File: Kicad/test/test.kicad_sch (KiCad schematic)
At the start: 74 parts, among them J1 SPKOUT, J2 Tag Con, P1 USB_C_Plug_USB2.0, SW1 SW_Push, SW2 SW_Push, SW4 SW_Push, SW5 SW_Push, U1 MAX98357A, U2 ESP32-S3-WROOM-1, U3 OV5640, U4 24Mhz, U5 AXP2101

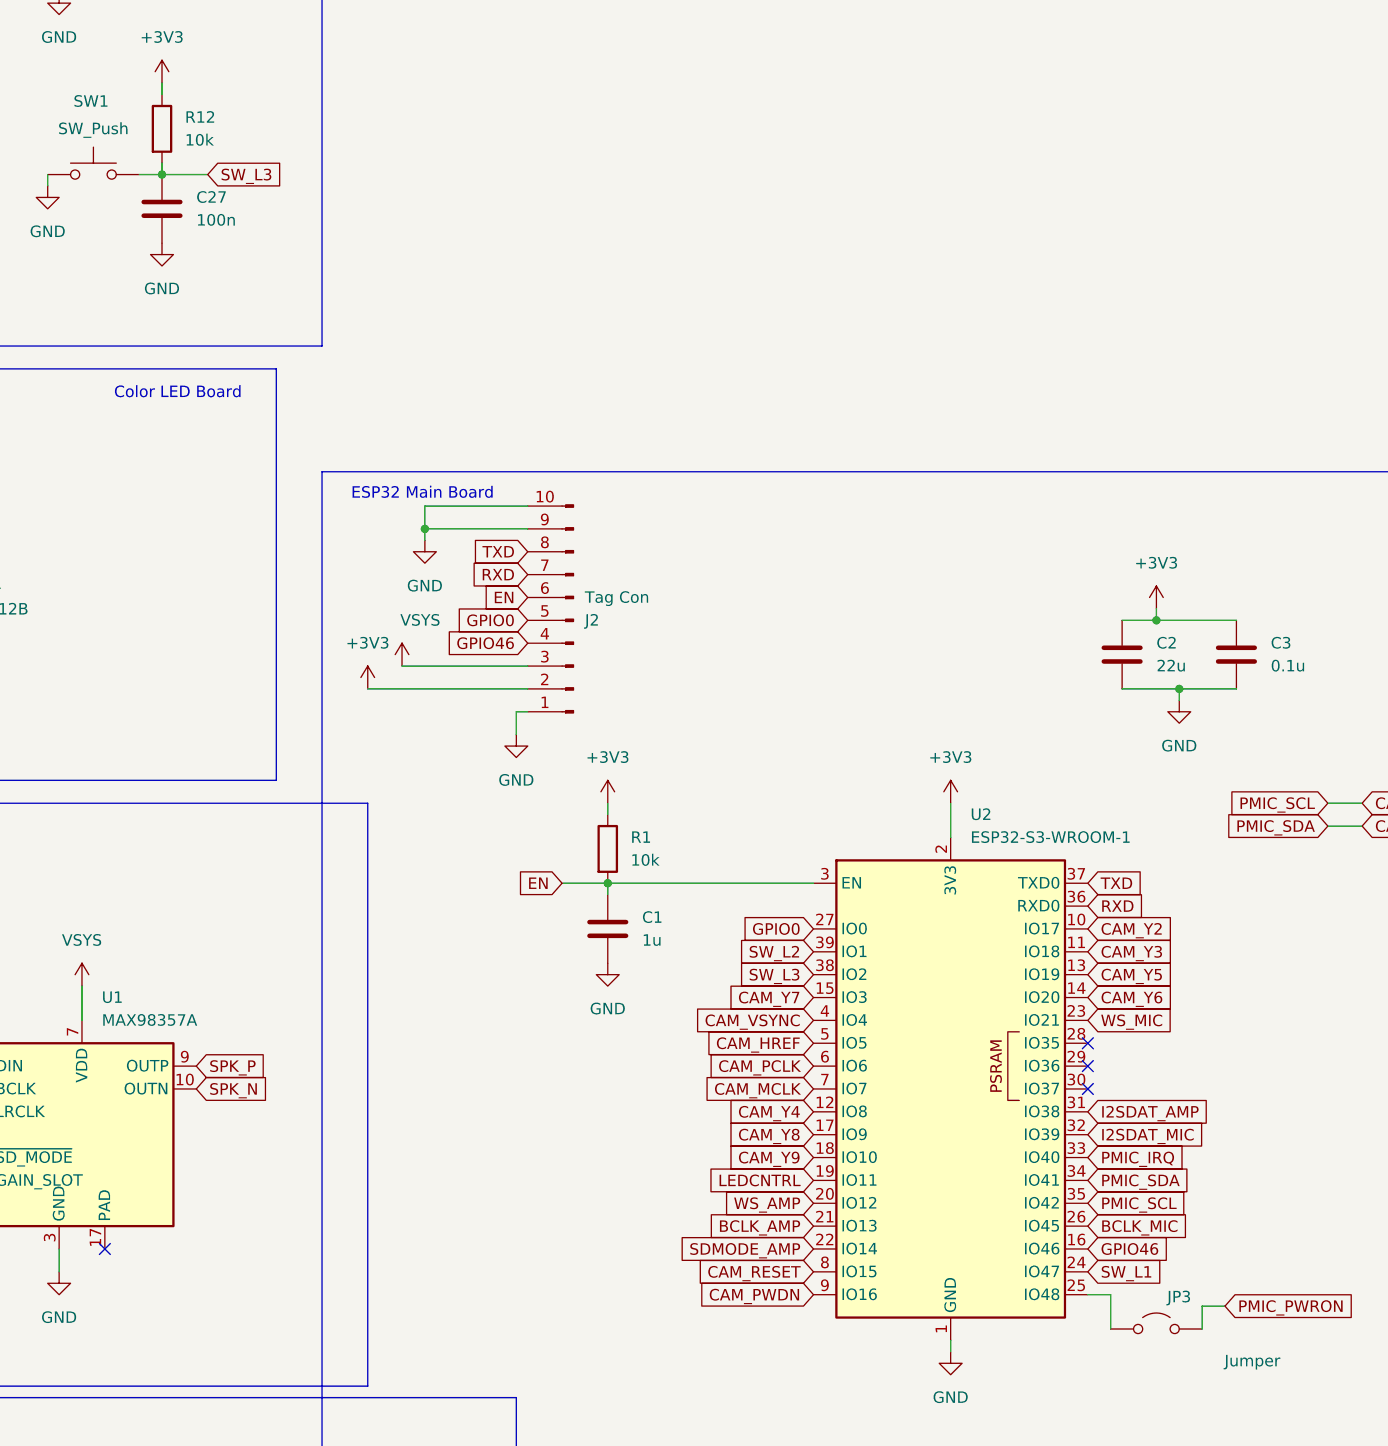
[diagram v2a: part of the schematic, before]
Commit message: ROUTED MORE
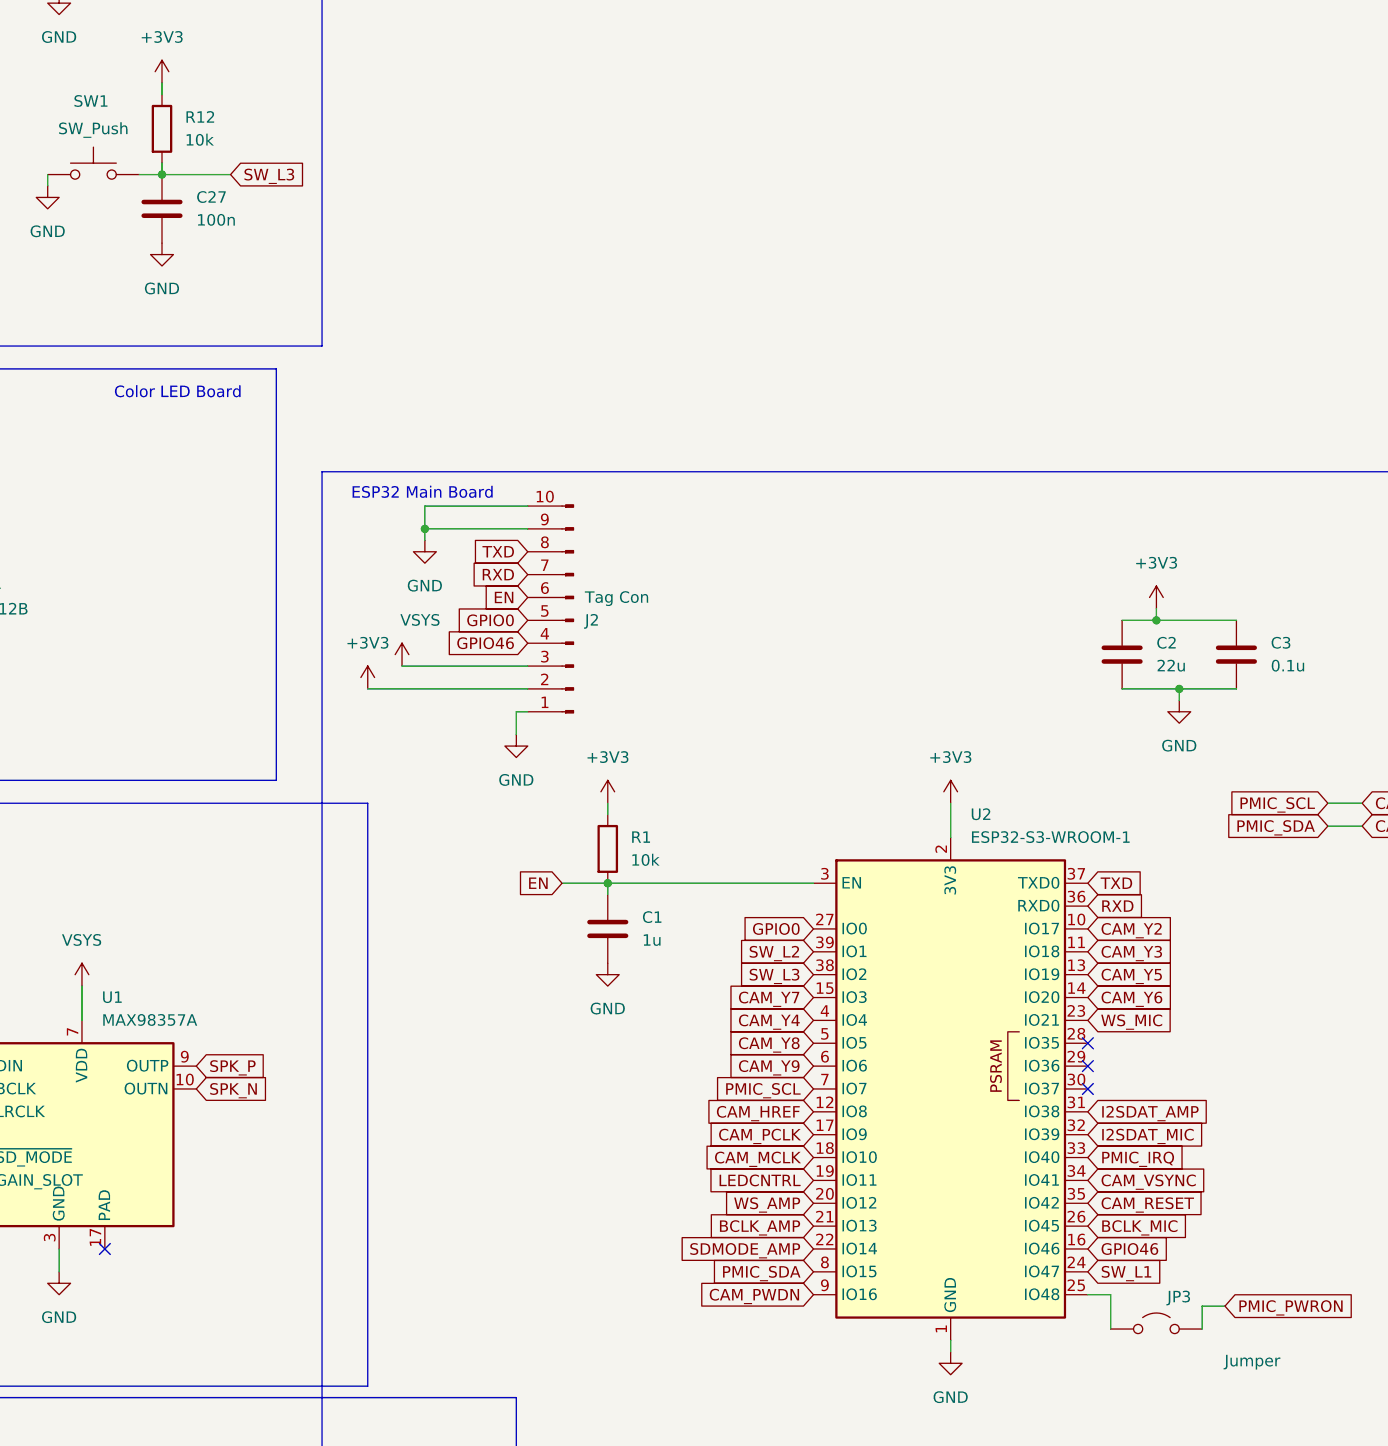
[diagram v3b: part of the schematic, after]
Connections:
- net CAM_HREF: now also U2.12 (IO8); no longer U2.5 (IO5)
- net CAM_MCLK: now also U2.18 (IO10); no longer U2.7 (IO7)
- net CAM_PCLK: now also U2.17 (IO9); no longer U2.6 (IO6)
- net CAM_RESET: now also U2.35 (IO42); no longer U2.8 (IO15)
- net CAM_SCL: now also U2.7 (IO7); no longer U2.35 (IO42)
- net CAM_SDA: now also U2.8 (IO15); no longer U2.34 (IO41)
- net CAM_VSYNC: now also U2.34 (IO41); no longer U2.4 (IO4)
- net CAM_Y4: now also U2.4 (IO4); no longer U2.12 (IO8)
- net CAM_Y8: now also U2.5 (IO5); no longer U2.17 (IO9)
- net CAM_Y9: now also U2.6 (IO6); no longer U2.18 (IO10)

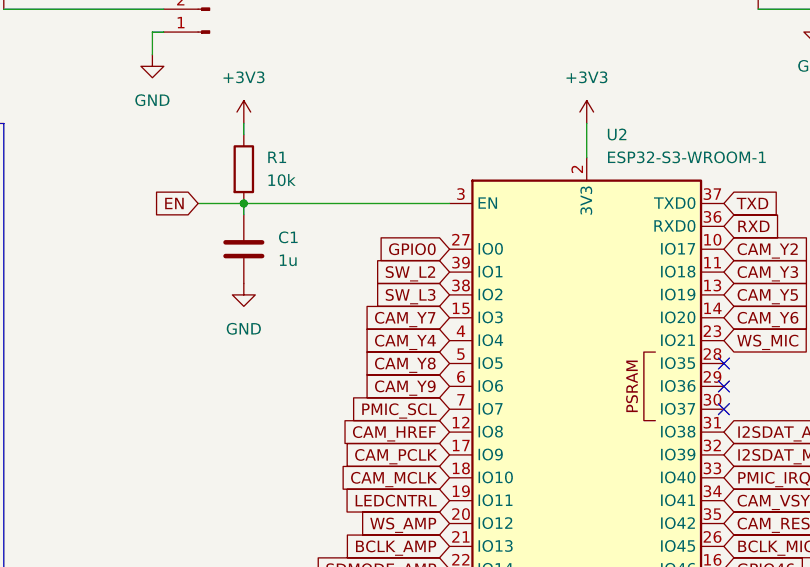
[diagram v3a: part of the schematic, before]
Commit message: Routing 80% Done
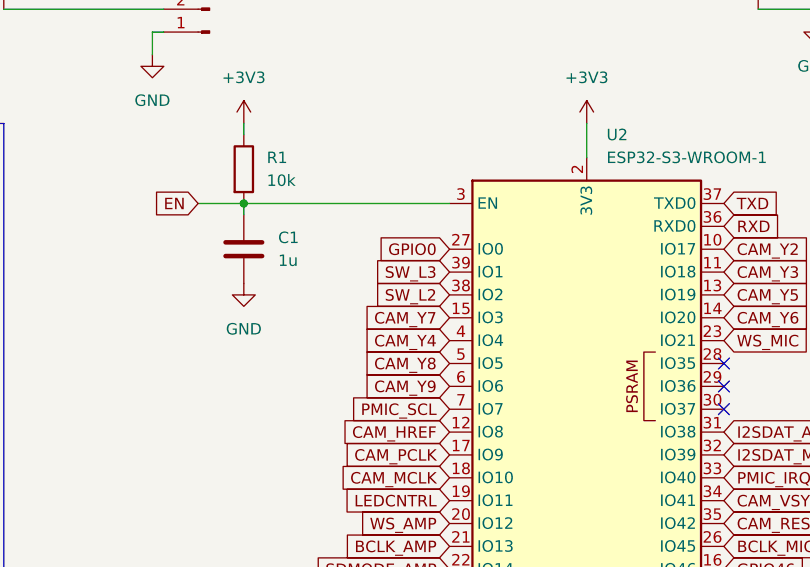
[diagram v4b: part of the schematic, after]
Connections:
- net SW_L2: now also U2.38 (IO2); no longer U2.39 (IO1)
- net SW_L3: now also U2.39 (IO1); no longer U2.38 (IO2)
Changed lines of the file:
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@@
 	(global_label "SW_L3"
 		(shape input)
+		(at 321.31 184.15 180)
+		(fields_autoplaced yes)
+		(effects
+			(font
+				(size 1.27 1.27)
+			)
+			(justify right)
+		)
+		(property "Intersheetrefs" "${INTERSHEET_REFS}"
+			(at 312.4587 184.15 0)
+			(effects
+				(font
+					(size 1.27 1.27)
+				)
+				(justify right)
+				(hide yes)
+			)
+		)
+	)
+	(global_label "PMIC_PWRON"
+		(shape input)
+		(at 248.92 69.85 0)
+		(fields_autoplaced yes)
+		(effects
+			(font
+				(size 1.27 1.27)
+			)
+			(justify left)
+		)
+		(property "Intersheetrefs" "${INTERSHEET_REFS}"
+			(at 264.1214 69.85 0)
+			(effects
+				(font
+					(size 1.27 1.27)
+				)
+				(justify left)
+				(hide yes)
+			)
+		)
+	)
+	(global_label "CAM_RESET"
+		(shape input)
+		(at 351.79 212.09 0)
+		(fields_autoplaced yes)
+		(effects
+			(font
+				(size 1.27 1.27)
+			)
+			(justify left)
+		)
+		(property "Intersheetrefs" "${INTERSHEET_REFS}"
+			(at 365.2979 212.09 0)
+			(effects
+				(font
+					(size 1.27 1.27)
+				)
+				(justify left)
+				(hide yes)
+			)
+		)
+	)
+	(global_label "CAM_VSYNC"
+		(shape input)
+		(at 351.79 209.55 0)
+		(fields_autoplaced yes)
+		(effects
+			(font
+				(size 1.27 1.27)
+			)
+			(justify left)
+		)
+		(property "Intersheetrefs" "${INTERSHEET_REFS}"
+			(at 365.54 209.55 0)
+			(effects
+				(font
+					(size 1.27 1.27)
+				)
+				(justify left)
+				(hide yes)
+			)
+		)
+	)
+	(global_label "I2SDAT_MIC"
+		(shape input)
+		(at 204.47 264.16 180)
+		(fields_autoplaced yes)
+		(effects
+			(font
+				(size 1.27 1.27)
+			)
+			(justify right)
+		)
+		(property "Intersheetrefs" "${INTERSHEET_REFS}"
+			(at 190.841 264.16 0)
+			(effects
+				(font
+					(size 1.27 1.27)
+				)
+				(justify right)
+				(hide yes)
+			)
+		)
+	)
+	(global_label "CAM_Y9"
+		(shape input)
+		(at 321.31 196.85 180)
+		(fields_autoplaced yes)
+		(effects
+			(font
+				(size 1.27 1.27)
+			)
+			(justify right)
+		)
+		(property "Intersheetrefs" "${INTERSHEET_REFS}"
+			(at 311.2491 196.85 0)
+			(effects
+				(font
+					(size 1.27 1.27)
+				)
+				(justify right)
+				(hide yes)
+			)
+		)
+	)
+	(global_label "CAM_Y4"
+		(shape input)
+		(at 83.82 251.46 180)
+		(fields_autoplaced yes)
+		(effects
+			(font
+				(size 1.27 1.27)
+			)
+			(justify right)
+		)
+		(property "Intersheetrefs" "${INTERSHEET_REFS}"
+			(at 73.7591 251.46 0)
+			(effects
+				(font
+					(size 1.27 1.27)
+				)
+				(justify right)
+				(hide yes)
+			)
+		)
+	)
+	(global_label "CAM_SDA"
+		(shape input)
+		(at 119.38 236.22 0)
+		(fields_autoplaced yes)
+		(effects
+			(font
+				(size 1.27 1.27)
+			)
+			(justify left)
+		)
+		(property "Intersheetrefs" "${INTERSHEET_REFS}"
+			(at 130.7109 236.22 0)
+			(effects
+				(font
+					(size 1.27 1.27)
+				)
+				(justify left)
+				(hide yes)
+			)
+		)
+	)
+	(global_label "CAM_CLKINTRNL"
+		(shape input)
+		(at 128.27 261.62 270)
+		(fields_autoplaced yes)
+		(effects
+			(font
+				(size 1.27 1.27)
+			)
+			(justify right)
+		)
+		(property "Intersheetrefs" "${INTERSHEET_REFS}"
+			(at 128.27 279.4824 90)
+			(effects
+				(font
+					(size 1.27 1.27)
+				)
+				(justify right)
+				(hide yes)
+			)
+		)
+	)
+	(global_label "PMIC_SDA"
+		(shape input)
+		(at 71.12 148.59 180)
+		(fields_autoplaced yes)
+		(effects
+			(font
+				(size 1.27 1.27)
+			)
+			(justify right)
+		)
+		(property "Intersheetrefs" "${INTERSHEET_REFS}"
+			(at 59.0029 148.59 0)
+			(effects
+				(font
+					(size 1.27 1.27)
+				)
+				(justify right)
+				(hide yes)
+			)
+		)
+	)
+	(global_label "LEDCNTRL"
+		(shape input)
+		(at 207.01 149.86 180)
+		(fields_autoplaced yes)
+		(effects
+			(font
+				(size 1.27 1.27)
+			)
+			(justify right)
+		)
+		(property "Intersheetrefs" "${INTERSHEET_REFS}"
+			(at 194.7115 149.86 0)
+			(effects
+				(font
+					(size 1.27 1.27)
+				)
+				(justify right)
+				(hide yes)
+			)
+		)
+	)
+	(global_label "SW_L2"
+		(shape input)
 		(at 321.31 186.69 180)
 		(fields_autoplaced yes)
@@
 			(effects
 				(font
-					(size 1.27 1.27)
-				)
-				(justify right)
-				(hide yes)
-			)
-		)
-	)
-	(global_label "PMIC_PWRON"
-		(shape input)
-		(at 248.92 69.85 0)
-		(fields_autoplaced yes)
-		(effects
-			(font
-				(size 1.27 1.27)
-			)
-			(justify left)
-		)
-		(property "Intersheetrefs" "${INTERSHEET_REFS}"
-			(at 264.1214 69.85 0)
-			(effects
-				(font
-					(size 1.27 1.27)
-				)
-				(justify left)
-				(hide yes)
-			)
-		)
-	)
-	(global_label "CAM_RESET"
-		(shape input)
-		(at 351.79 212.09 0)
-		(fields_autoplaced yes)
-		(effects
-			(font
-				(size 1.27 1.27)
-			)
-			(justify left)
-		)
-		(property "Intersheetrefs" "${INTERSHEET_REFS}"
-			(at 365.2979 212.09 0)
-			(effects
-				(font
-					(size 1.27 1.27)
-				)
-				(justify left)
-				(hide yes)
-			)
-		)
-	)
-	(global_label "CAM_VSYNC"
-		(shape input)
-		(at 351.79 209.55 0)
-		(fields_autoplaced yes)
-		(effects
-			(font
-				(size 1.27 1.27)
-			)
-			(justify left)
-		)
-		(property "Intersheetrefs" "${INTERSHEET_REFS}"
-			(at 365.54 209.55 0)
-			(effects
-				(font
-					(size 1.27 1.27)
-				)
-				(justify left)
-				(hide yes)
-			)
-		)
-	)
-	(global_label "I2SDAT_MIC"
-		(shape input)
-		(at 204.47 264.16 180)
-		(fields_autoplaced yes)
-		(effects
-			(font
-				(size 1.27 1.27)
-			)
-			(justify right)
-		)
-		(property "Intersheetrefs" "${INTERSHEET_REFS}"
-			(at 190.841 264.16 0)
-			(effects
-				(font
-					(size 1.27 1.27)
-				)
-				(justify right)
-				(hide yes)
-			)
-		)
-	)
-	(global_label "CAM_Y9"
-		(shape input)
-		(at 321.31 196.85 180)
-		(fields_autoplaced yes)
-		(effects
-			(font
-				(size 1.27 1.27)
-			)
-			(justify right)
-		)
-		(property "Intersheetrefs" "${INTERSHEET_REFS}"
-			(at 311.2491 196.85 0)
-			(effects
-				(font
-					(size 1.27 1.27)
-				)
-				(justify right)
-				(hide yes)
-			)
-		)
-	)
-	(global_label "CAM_Y4"
-		(shape input)
-		(at 83.82 251.46 180)
-		(fields_autoplaced yes)
-		(effects
-			(font
-				(size 1.27 1.27)
-			)
-			(justify right)
-		)
-		(property "Intersheetrefs" "${INTERSHEET_REFS}"
-			(at 73.7591 251.46 0)
-			(effects
-				(font
-					(size 1.27 1.27)
-				)
-				(justify right)
-				(hide yes)
-			)
-		)
-	)
-	(global_label "CAM_SDA"
-		(shape input)
-		(at 119.38 236.22 0)
-		(fields_autoplaced yes)
-		(effects
-			(font
-				(size 1.27 1.27)
-			)
-			(justify left)
-		)
-		(property "Intersheetrefs" "${INTERSHEET_REFS}"
-			(at 130.7109 236.22 0)
-			(effects
-				(font
-					(size 1.27 1.27)
-				)
-				(justify left)
-				(hide yes)
-			)
-		)
-	)
-	(global_label "CAM_CLKINTRNL"
-		(shape input)
-		(at 128.27 261.62 270)
-		(fields_autoplaced yes)
-		(effects
-			(font
-				(size 1.27 1.27)
-			)
-			(justify right)
-		)
-		(property "Intersheetrefs" "${INTERSHEET_REFS}"
-			(at 128.27 279.4824 90)
-			(effects
-				(font
-					(size 1.27 1.27)
-				)
-				(justify right)
-				(hide yes)
-			)
-		)
-	)
-	(global_label "PMIC_SDA"
-		(shape input)
-		(at 71.12 148.59 180)
-		(fields_autoplaced yes)
-		(effects
-			(font
-				(size 1.27 1.27)
-			)
-			(justify right)
-		)
-		(property "Intersheetrefs" "${INTERSHEET_REFS}"
-			(at 59.0029 148.59 0)
-			(effects
-				(font
-					(size 1.27 1.27)
-				)
-				(justify right)
-				(hide yes)
-			)
-		)
-	)
-	(global_label "LEDCNTRL"
-		(shape input)
-		(at 207.01 149.86 180)
-		(fields_autoplaced yes)
-		(effects
-			(font
-				(size 1.27 1.27)
-			)
-			(justify right)
-		)
-		(property "Intersheetrefs" "${INTERSHEET_REFS}"
-			(at 194.7115 149.86 0)
-			(effects
-				(font
-					(size 1.27 1.27)
-				)
-				(justify right)
-				(hide yes)
-			)
-		)
-	)
-	(global_label "SW_L2"
-		(shape input)
-		(at 321.31 184.15 180)
-		(fields_autoplaced yes)
-		(effects
-			(font
-				(size 1.27 1.27)
-			)
-			(justify right)
-		)
-		(property "Intersheetrefs" "${INTERSHEET_REFS}"
-			(at 312.4587 184.15 0)
-			(effects
-				(font

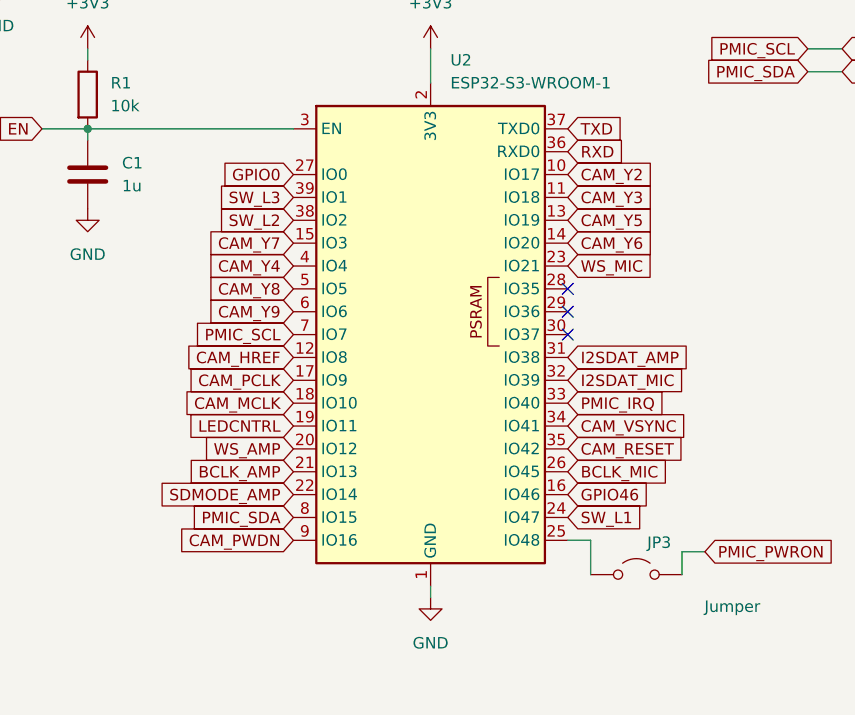
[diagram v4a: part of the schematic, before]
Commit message: Routing 95% done
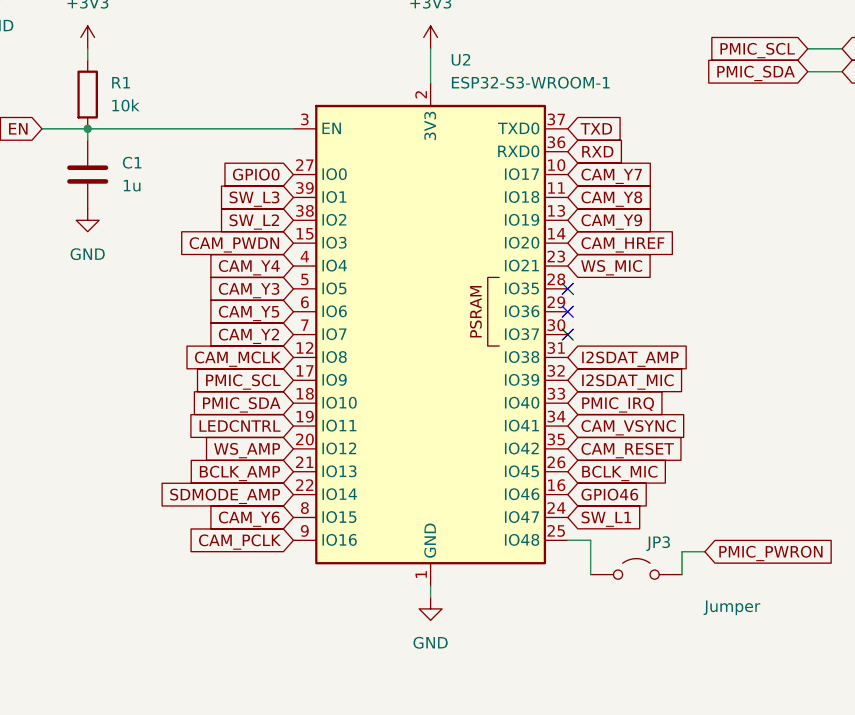
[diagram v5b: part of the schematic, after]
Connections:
- net CAM_HREF: now also U2.14 (IO20); no longer U2.12 (IO8)
- net CAM_MCLK: now also U2.12 (IO8); no longer U2.18 (IO10)
- net CAM_PCLK: now also U2.9 (IO16); no longer U2.17 (IO9)
- net CAM_PWDN: now also U2.15 (IO3); no longer U2.9 (IO16)
- net CAM_SCL: now also U2.17 (IO9); no longer U2.7 (IO7)
- net CAM_SDA: now also U2.18 (IO10); no longer U2.8 (IO15)
- net CAM_Y2: now also U2.7 (IO7); no longer U2.10 (IO17)
- net CAM_Y3: now also U2.5 (IO5); no longer U2.11 (IO18)
- net CAM_Y5: now also U2.6 (IO6); no longer U2.13 (IO19)
- net CAM_Y6: now also U2.8 (IO15); no longer U2.14 (IO20)
- net CAM_Y7: now also U2.10 (IO17); no longer U2.15 (IO3)
- net CAM_Y8: now also U2.11 (IO18); no longer U2.5 (IO5)
- net CAM_Y9: now also U2.13 (IO19); no longer U2.6 (IO6)
